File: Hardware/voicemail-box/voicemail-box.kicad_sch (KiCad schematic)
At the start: 0 parts

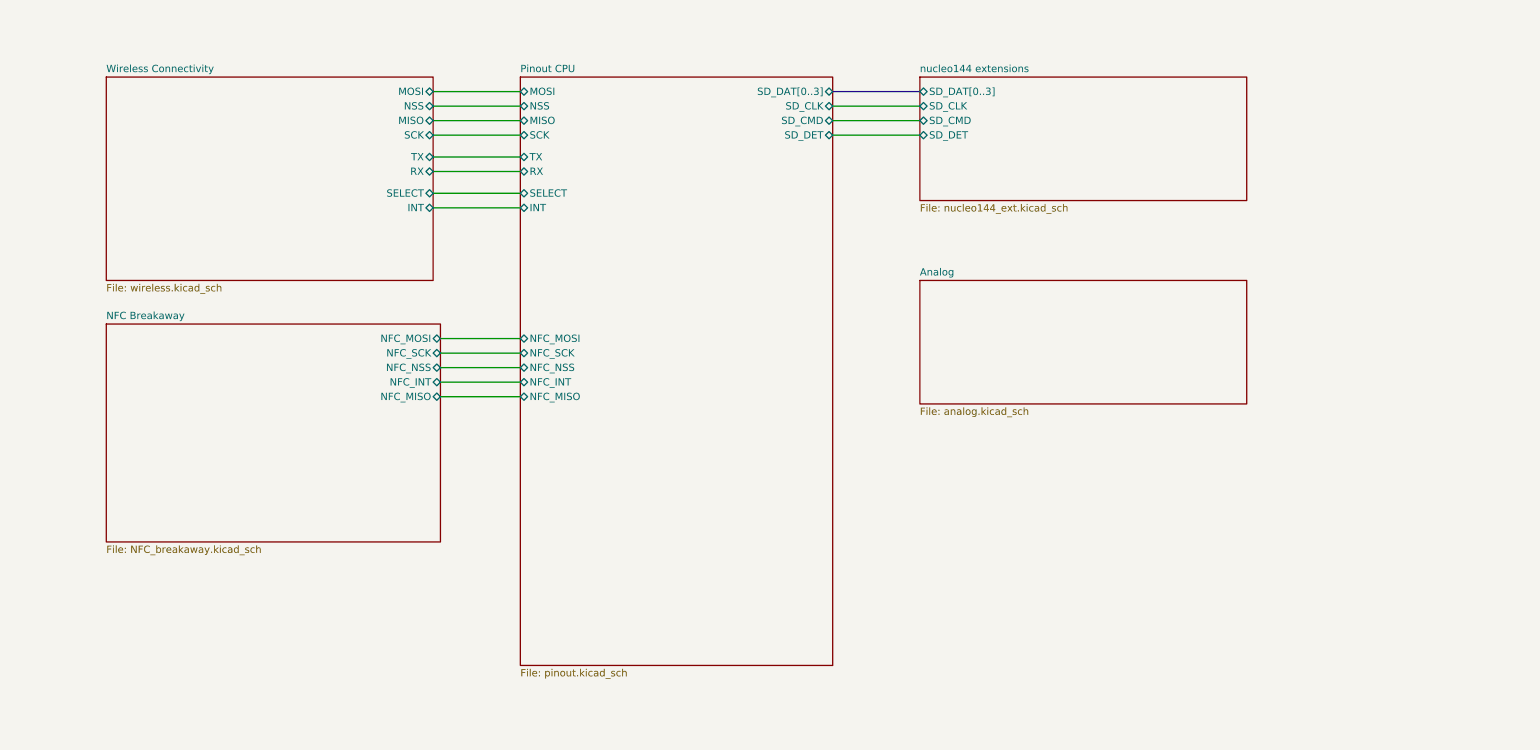
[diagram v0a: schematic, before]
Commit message: -
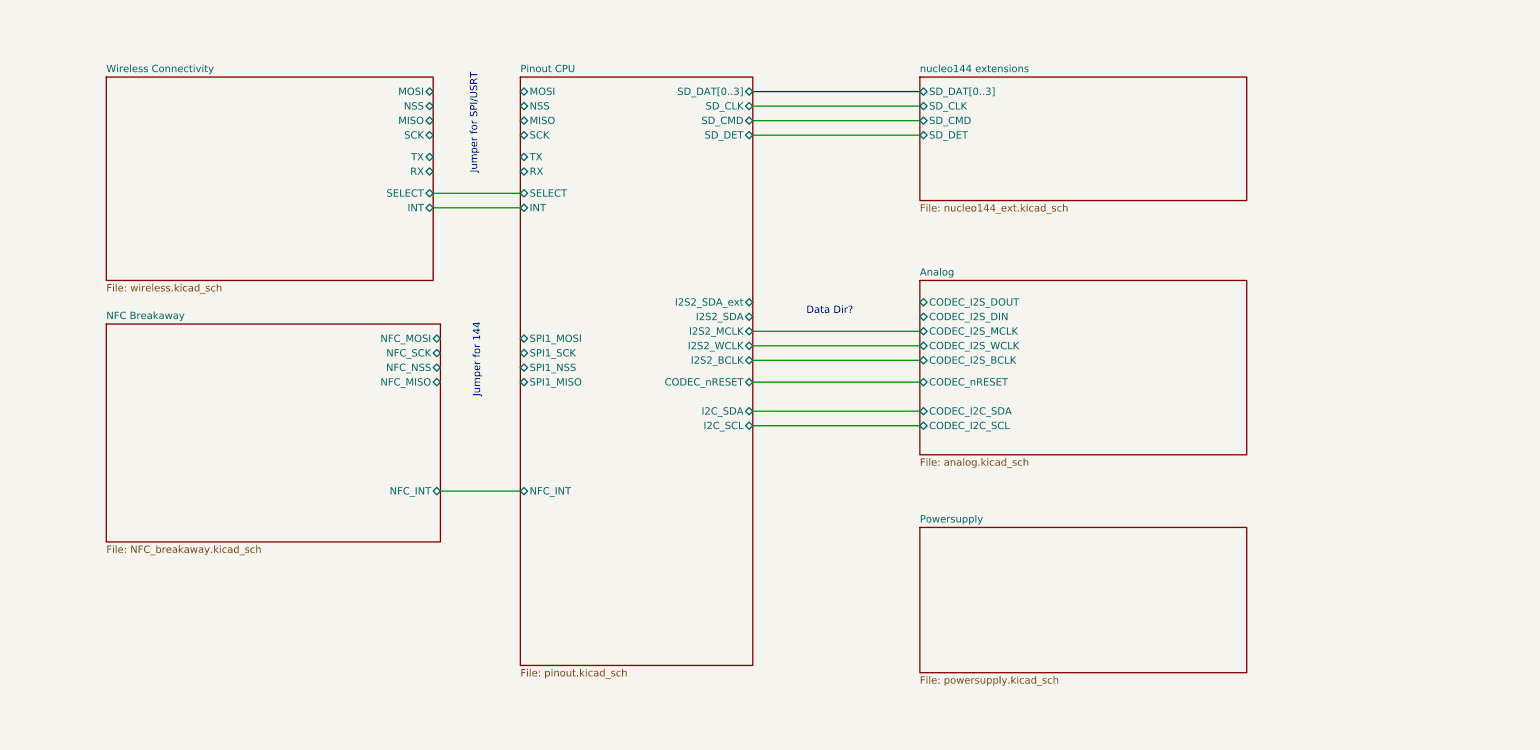
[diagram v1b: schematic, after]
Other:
- added sheet Powersupply (powersupply.kicad_sch)
- sheet Analog ports: added CODEC_I2C_SCL, CODEC_I2C_SDA, CODEC_I2S_BCLK, CODEC_I2S_DIN, CODEC_I2S_DOUT, CODEC_I2S_MCLK, CODEC_I2S_WCLK, CODEC_nRESET; removed none
- sheet Pinout CPU ports: added CODEC_nRESET, I2C_SCL, I2C_SDA, I2S2_BCLK, I2S2_MCLK, I2S2_SDA, I2S2_SDA_ext, I2S2_WCLK, SPI1_MISO, SPI1_MOSI, SPI1_NSS, SPI1_SCK; removed NFC_MISO, NFC_MOSI, NFC_NSS, NFC_SCK
- note added: "Data Dir?"
- note added: "Jumper for 144"
- note added: "Jumper for SPI/USRT"

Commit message: schematic draft
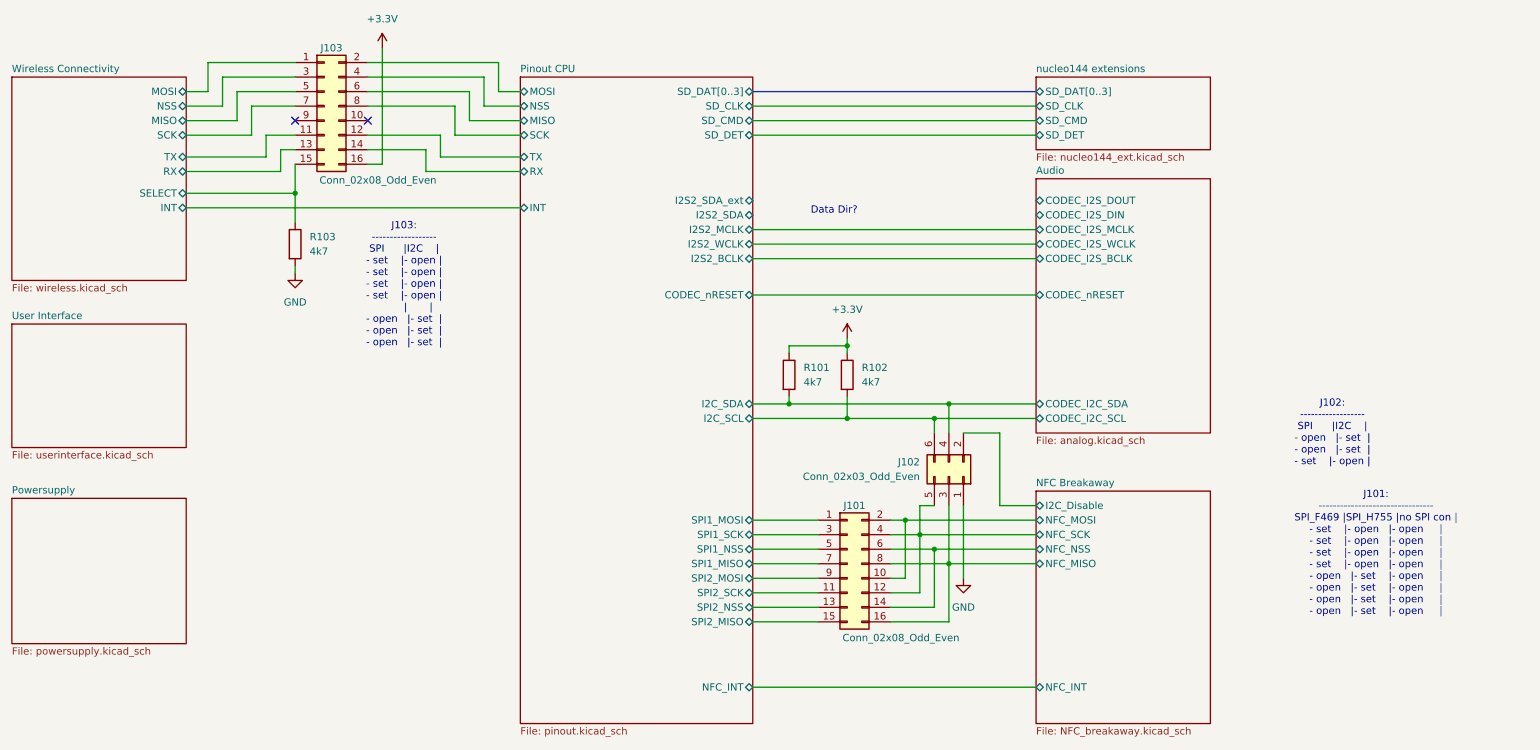
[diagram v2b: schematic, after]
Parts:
- added J101, J103: Conn_02x08_Odd_Even, Connector_PinHeader_2.54mm:PinHeader_2x08_P2.54mm_Vertical, symbol Connector_Generic:Conn_02x08_Odd_Even
- added J102: Conn_02x03_Odd_Even, Connector_PinSocket_2.54mm:PinSocket_2x03_P2.54mm_Vertical, symbol Connector_Generic:Conn_02x03_Odd_Even
- added R101, R102, R103: 4k7, PCM_4ms_Resistor:R_0603, symbol Device:R
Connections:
- net Audio/CODEC_I2C_SCL: now also J102.6 (Pin_6), R102.2
- net Audio/CODEC_I2C_SDA: now also J102.4 (Pin_4), R101.2
- net NFC Breakaway/NFC_MISO: now also J101.16 (Pin_16), J101.8 (Pin_8), J102.3 (Pin_3)
- net NFC Breakaway/NFC_MOSI: now also J101.10 (Pin_10), J101.2 (Pin_2)
- net NFC Breakaway/NFC_NSS: now also J101.14 (Pin_14), J101.6 (Pin_6)
- net NFC Breakaway/NFC_SCK: now also J101.12 (Pin_12), J101.4 (Pin_4), J102.5 (Pin_5)
- net Pinout CPU/MISO: now also J103.6 (Pin_6)
- net Pinout CPU/MOSI: now also J103.2 (Pin_2)
- net Pinout CPU/NSS: now also J103.4 (Pin_4)
- net Pinout CPU/RX: now also J103.14 (Pin_14)
- net Pinout CPU/SCK: now also J103.8 (Pin_8)
- net Pinout CPU/SPI1_MISO: now also J101.7 (Pin_7)
- net Pinout CPU/SPI1_MOSI: now also J101.1 (Pin_1)
- net Pinout CPU/SPI1_NSS: now also J101.5 (Pin_5)
- net Pinout CPU/SPI1_SCK: now also J101.3 (Pin_3)
- net Pinout CPU/TX: now also J103.12 (Pin_12)
- net Wireless Connectivity/MISO: now also J103.5 (Pin_5)
- net Wireless Connectivity/MOSI: now also J103.1 (Pin_1)
- net Wireless Connectivity/NSS: now also J103.3 (Pin_3)
- net Wireless Connectivity/RX: now also J103.13 (Pin_13)
- net Wireless Connectivity/SCK: now also J103.7 (Pin_7)
- net Wireless Connectivity/TX: now also J103.11 (Pin_11)
- new net +3.3V: J103.16 (Pin_16), R101.1, R102.1
- new net GND: J102.1 (Pin_1), R103.2
- new net NFC Breakaway/I2C_Disable: J102.2 (Pin_2)
- new net Pinout CPU/SPI2_MISO: J101.15 (Pin_15)
- new net Pinout CPU/SPI2_MOSI: J101.9 (Pin_9)
- new net Pinout CPU/SPI2_NSS: J101.13 (Pin_13)
- new net Pinout CPU/SPI2_SCK: J101.11 (Pin_11)
- new net Wireless Connectivity/SELECT: J103.15 (Pin_15), R103.1
- no-connect marks 0 -> 2
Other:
- sheet Analog renamed Audio
- added sheet User Interface (userinterface.kicad_sch)
- sheet NFC Breakaway ports: added I2C_Disable; removed none
- sheet Pinout CPU ports: added SPI2_MISO, SPI2_MOSI, SPI2_NSS, SPI2_SCK; removed SELECT
- note added: "J101: -------------------------------- SPI_F469 |SPI_H755 |no SPI con | - set |- open |- open | - set |- open |- open | - set |- open |- open | - set |- open |- open | - open |- set |- open | - open |- set |- open | - open |- set |- open | - open |- set |- open |"
- note added: "J102: ------------------ SPI |I2C | - open |- set | - open |- set | - set |- open |"
- note added: "J103: ------------------ SPI |I2C | - set |- open | - set |- open | - set |- open | - set |- open | | | - open |- set | - open |- set | - open |- set |"
- note removed: "Jumper for 144"
- note removed: "Jumper for SPI/USRT"
